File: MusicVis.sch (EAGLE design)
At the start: 14 parts, among them J1 AUDIO_JACK_3.5MM_PTH

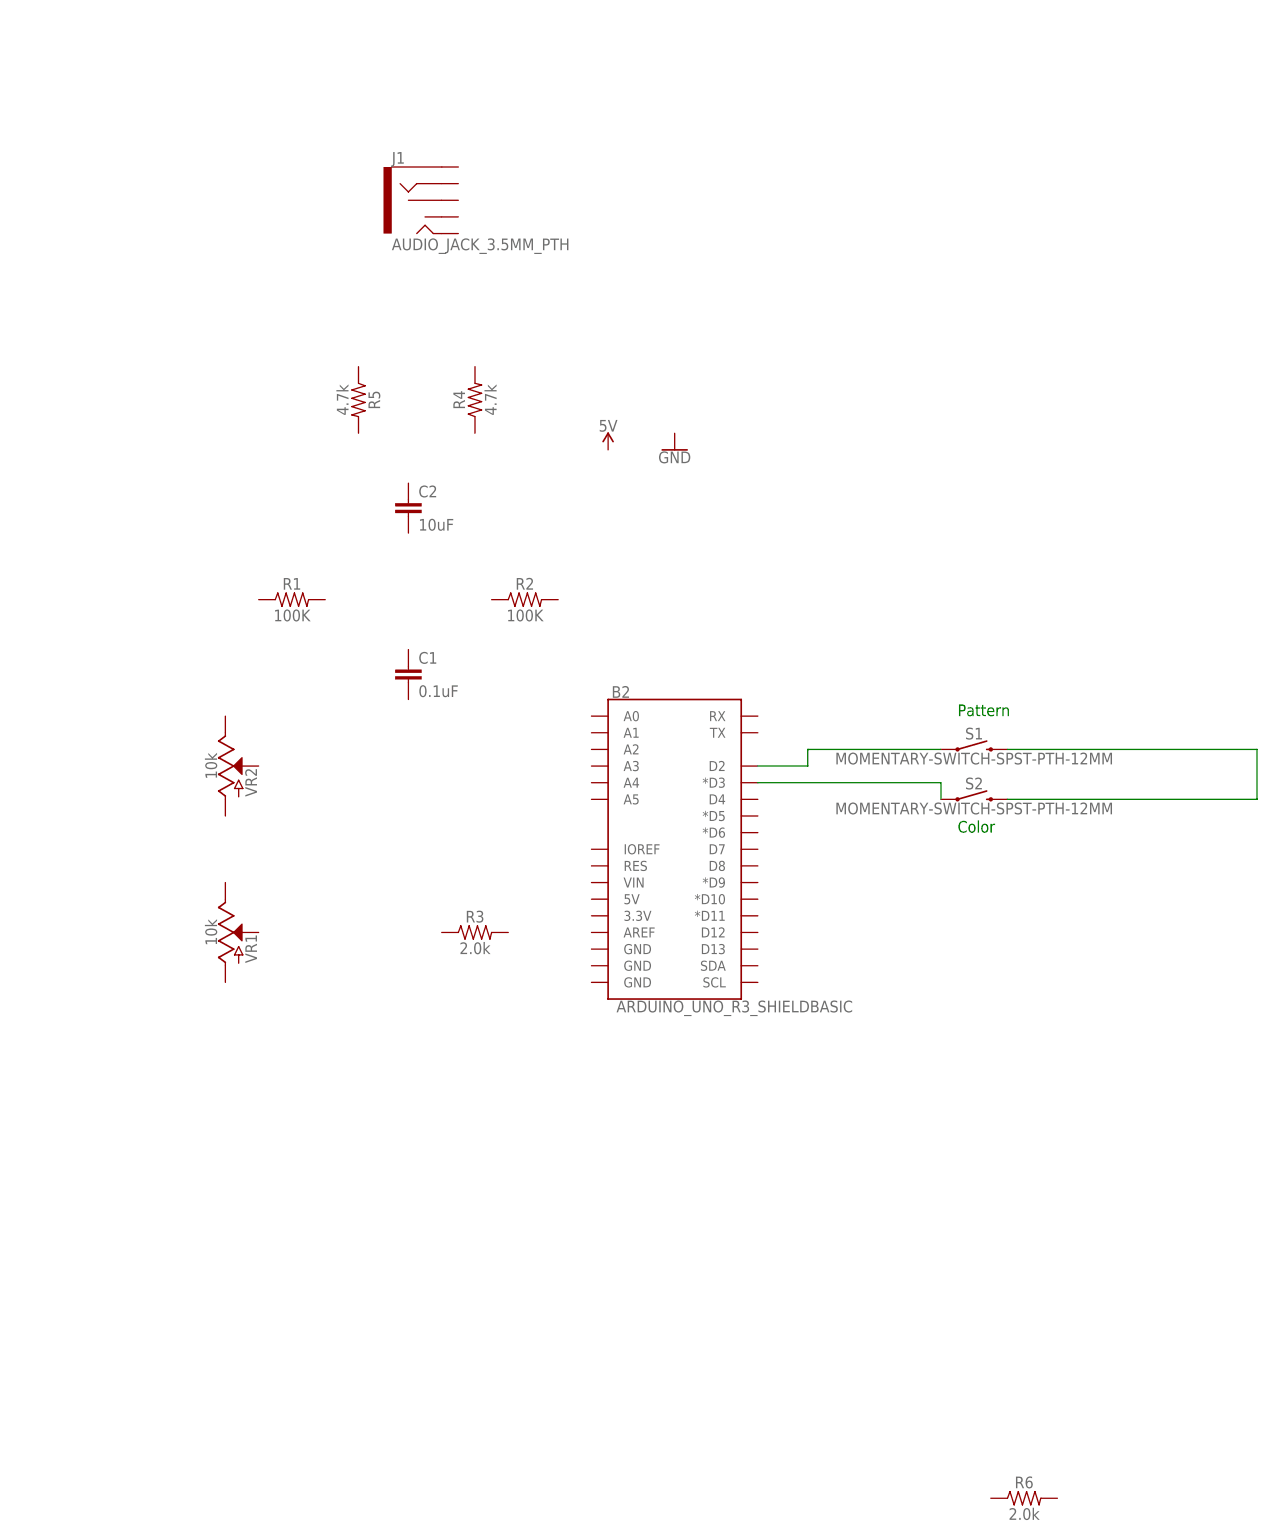
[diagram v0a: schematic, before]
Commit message: First pcd layout
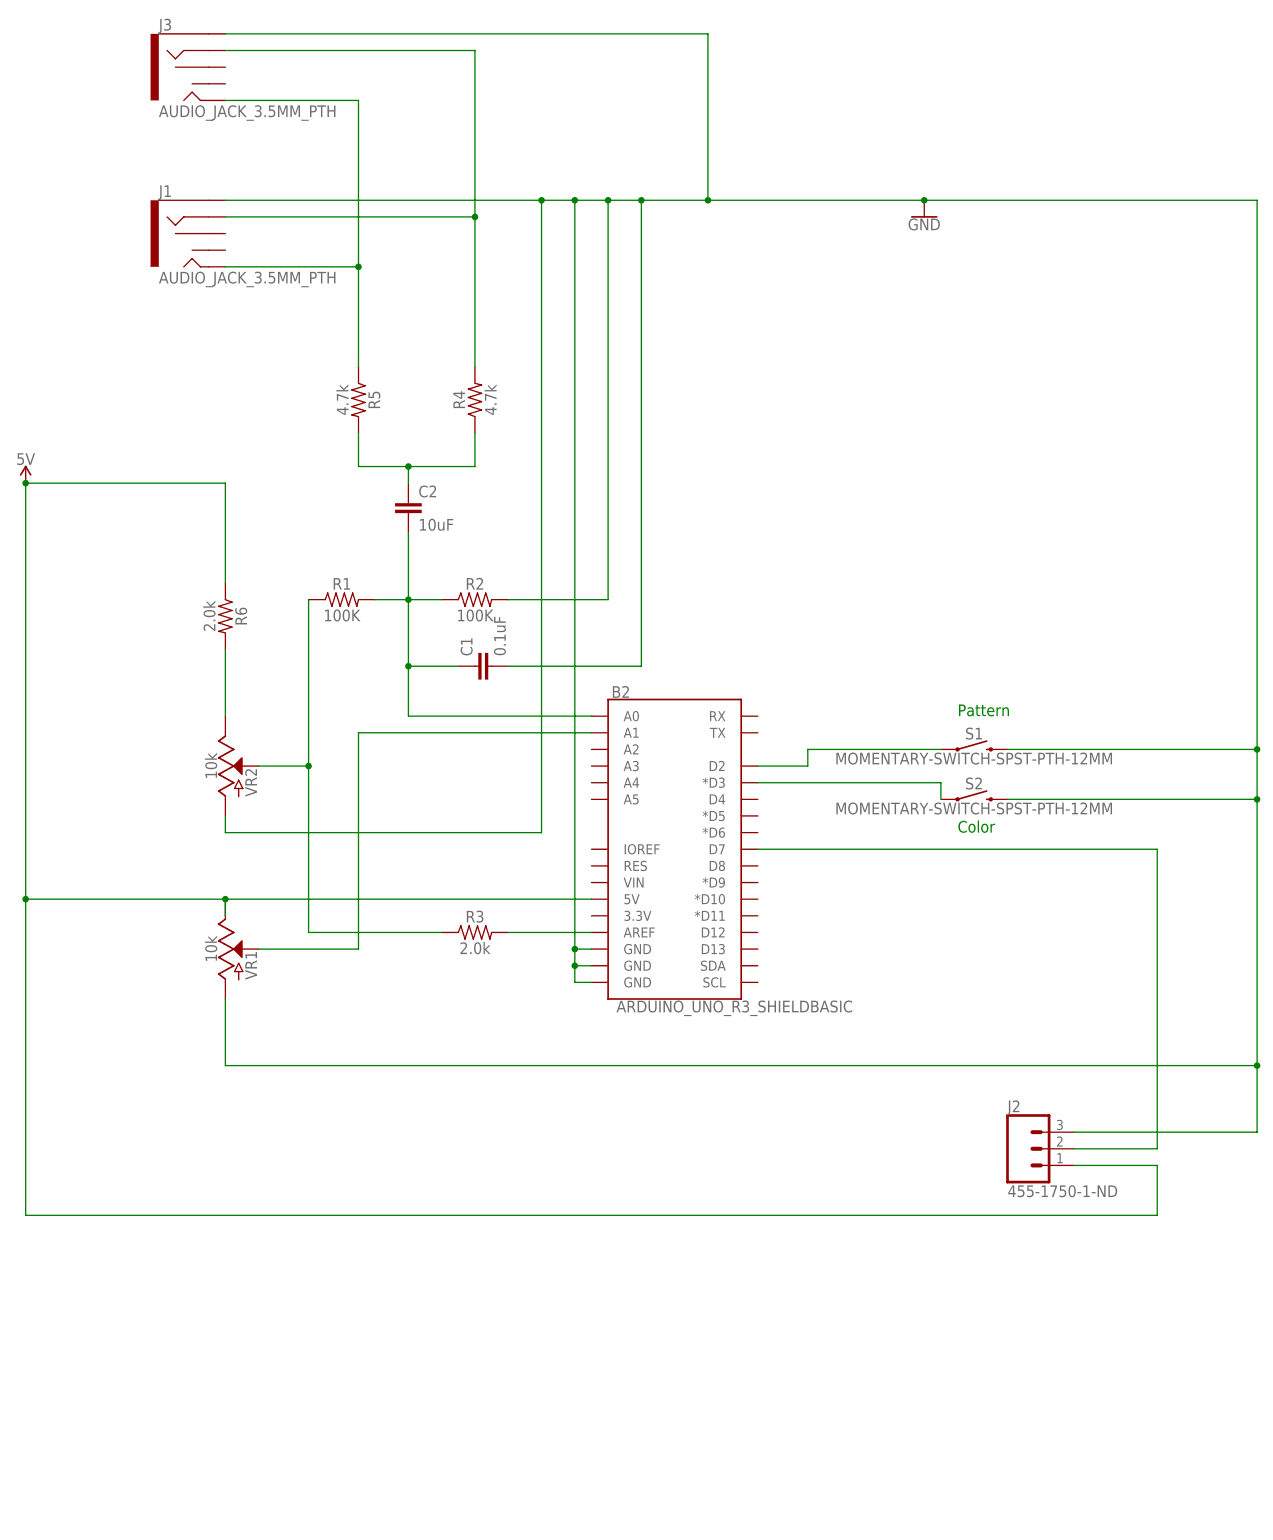
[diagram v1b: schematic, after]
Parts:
- added J2: 455-1750-1-ND, SparkFun-Connectors:CONN_03
- added J3: AUDIO_JACK_3.5MM_PTH, SparkFun-Connectors:AUDIO_JACK_3.5MM_PTH
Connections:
- new net 5V: B2.5V, J2.1, R6.1, VR1.E
- new net GND: B2.GND@0, B2.GND@1, B2.GND@2, C1.2, J1.SLEEVE, J2.3, J3.SLEEVE, R2.2, S1.2, S2.2, VR1.A, VR2.A
- new net N$11: B2.AREF, R3.2
- new net N$12: R1.1, R3.1, VR2.S
- new net N$14: B2.A1, VR1.S
- new net N$4: J1.TIP, J3.TIP, R5.1
- new net N$5: J1.RING, J3.RING, R4.2
- new net N$6: C2.1, R4.1, R5.2
- new net N$7: R6.2, VR2.E
- new net N$9: B2.A0, C1.1, C2.2, R1.2, R2.1
- net N$3: now also B2.D7, J2.2; no longer S1.2, S2.2
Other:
- moved on the sheet: C1, J1, R1, R2, R6, VR1
